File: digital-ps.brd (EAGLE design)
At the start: 73.7 x 50.8 mm, 85 parts, among them CON1 SWD_CON, IC1 STM32F334K8, IC2 MCP14700, IC3 7805, IC4 7805, IC5 3.3V, Q1 40V, Q2 40V, X1 12MHz

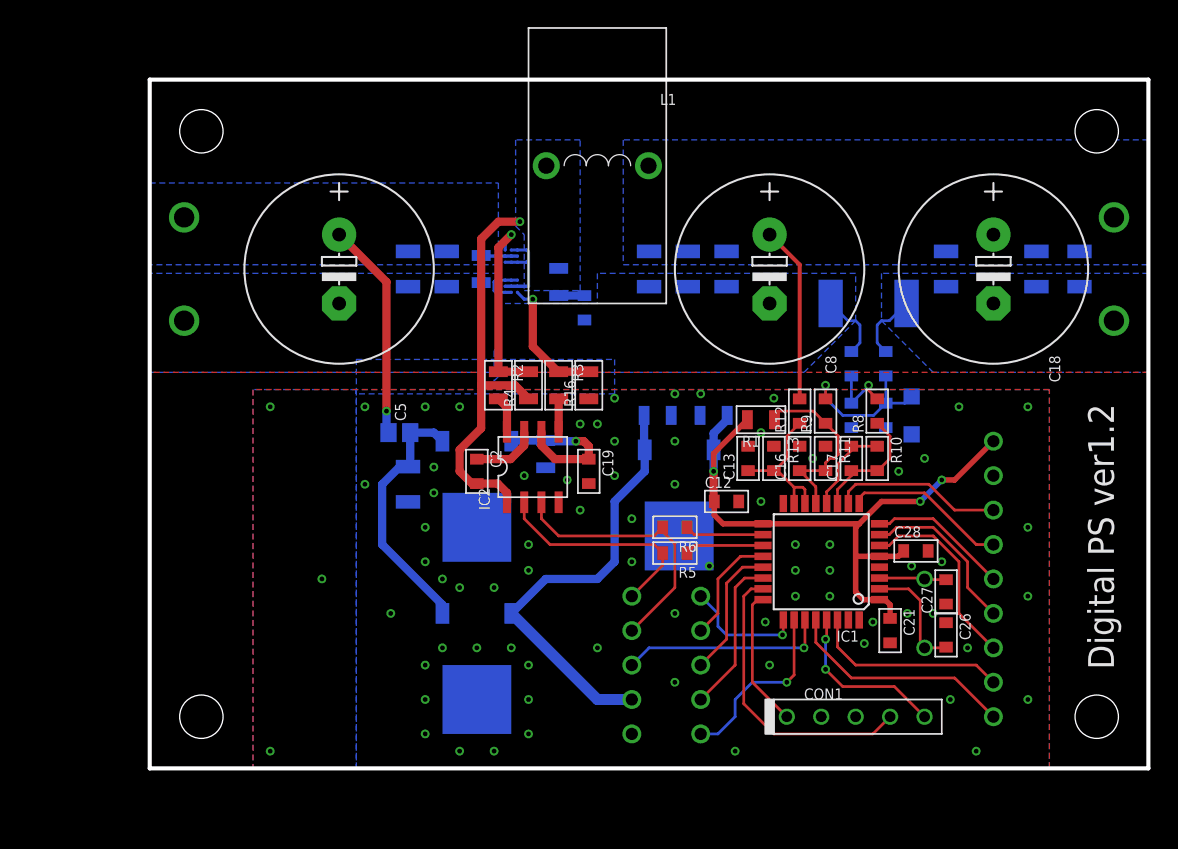
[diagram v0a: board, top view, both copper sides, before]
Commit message: 微修正
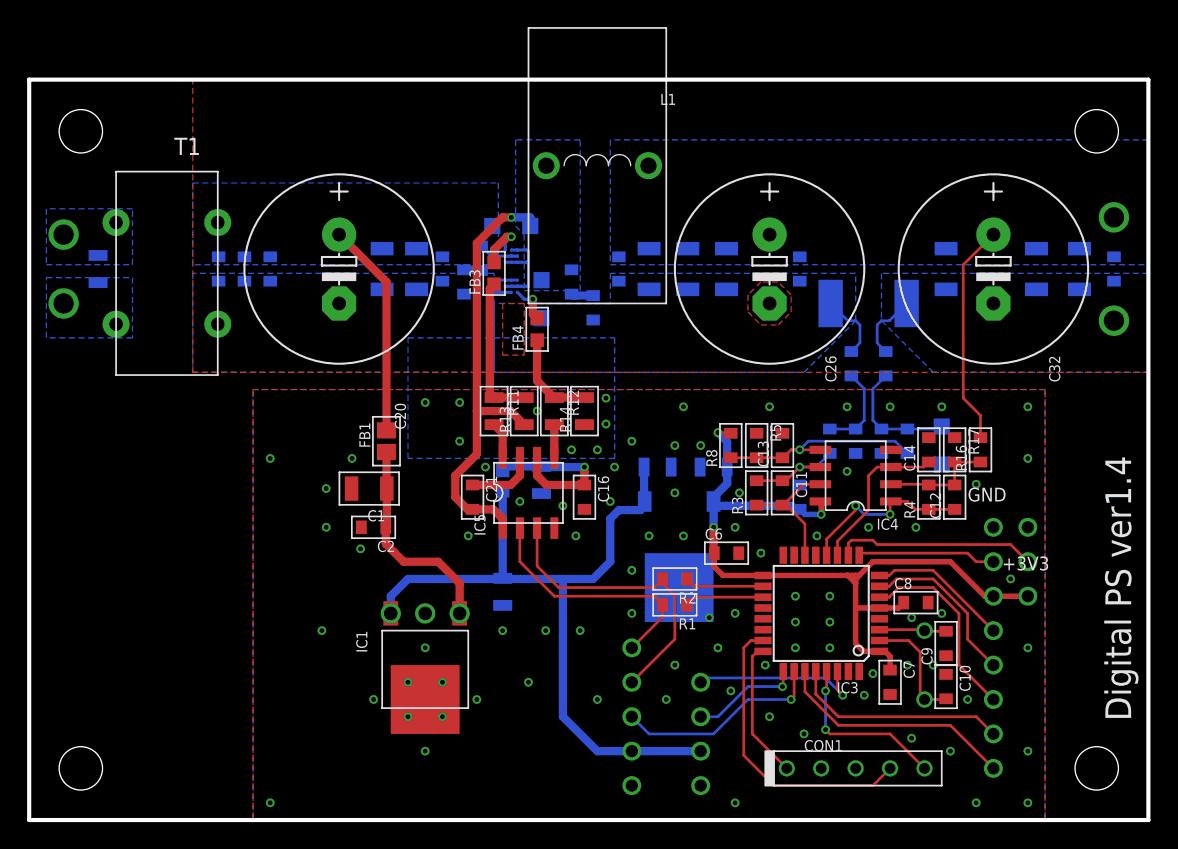
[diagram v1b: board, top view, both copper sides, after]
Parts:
- removed TP12: PA12, my_connector:TESTPIN
- removed TP13: PA11, my_connector:TESTPIN
- removed TP14: PA10, my_connector:TESTPIN
- added C30, C31, C33, C34: 10u, my_rcl:3225-2
- added C32: DNP, my_rcl:E5-13
- added C35, C36, C37, C39, C40: 1u, my_rcl:1608-2
- added C38: 0.1u, my_rcl:1608-2
- added C41: 1u, my_rcl:2012-2
- added D2, D3: SBD-1A2, my_rcl:SOD123
- added FB2: FB, my_rcl:1608-J
- added FB3, FB4: FB, my_rcl:1608-FB
- added R18: 10m, my_rcl:6432
- added R19: 2, my_rcl:1608-2
- added T1: COMMON_FILTER-SMALL, my_rcl:COMMON_FILTER__SMALL
- added TP24: +3V3, my_connector:TESTPIN
- added TP25, TP27: GND, my_connector:TESTPIN
- added TP26: +5V, my_connector:TESTPIN
- C1: device my_rcl:2012 -> my_rcl:3216
- C10, C9: value 10u -> 10p; device my_rcl:3216 -> my_rcl:1608
- C11: value 10u -> 1000p; device my_rcl:3216 -> my_rcl:1608
- C12: value 0.1u -> 1000p
- C15: value 1000p -> 10u; device my_rcl:1608 -> my_rcl:2012
- C16: value 1000p -> 0.1u
- C18: value DNP -> 1000p; device my_rcl:E5-13 -> my_rcl:1608
- C20: value 10u -> 1000u; device my_rcl:3216 -> my_rcl:E5-13
- C22, C23: device my_rcl:3216 -> my_rcl:3225-2
- C24: value 10u -> 1u; device my_rcl:3216 -> my_rcl:1608-2
- C25: value 10u -> 1n; device my_rcl:3216 -> my_rcl:1608-2
- C26: value 10p -> DNP; device my_rcl:1608 -> my_rcl:E5-13
- C27: value 10p -> 1u; device my_rcl:1608 -> my_rcl:1608-2
- C28: value 0.1u -> 10u; device my_rcl:1608 -> my_rcl:3225-2
- C29: value 1n -> 10u; device my_rcl:1608 -> my_rcl:3225-2
- C5: value 1000u -> 10u; device my_rcl:E5-13 -> my_rcl:2012
- C6: value 1u -> 0.1u; device my_rcl:2012 -> my_rcl:1608
- C7: value 10u -> 0.1u; device my_rcl:3216 -> my_rcl:1608
- C8: value DNP -> 0.1u; device my_rcl:E5-13 -> my_rcl:1608
- IC1: value STM32F334K8 -> 7805; device my_ic:TQFP32-08 -> my_ic:TO220-SOP-DUAL
- IC2: value MCP14700 -> 3.3V; device my_ic:SOP8 -> my_ic:P-HSIP3_2.30A
- IC3: value 7805 -> STM32F334K8; device my_ic:P-HSIP3_2.30A -> my_ic:TQFP32-08
- IC4: value 7805 -> OPA; device my_ic:P-HSIP3_2.30A -> my_ic:SOP8
- IC5: value 3.3V -> MCP14700; device my_ic:P-HSIP3_2.30A -> my_ic:SOP8
- Q1, Q2: value 40V -> EPC2052
- R1: value 1M -> 120; device my_rcl:2012 -> my_rcl:1608
- R10: value 10k -> 100
- R11, R12: value 10k -> 10; device my_rcl:1608 -> my_rcl:2012
- R13: value 1k -> 10k; device my_rcl:1608 -> my_rcl:2012
- R14: value 100 -> 10k; device my_rcl:1608 -> my_rcl:2012
- R15: value 100 -> 10; device my_rcl:1608 -> my_rcl:1608-2
- R16, R4: device my_rcl:2012 -> my_rcl:1608
- R17: value 10 -> 1k; device my_rcl:2012 -> my_rcl:1608
- R2: value 10 -> 120; device my_rcl:2012 -> my_rcl:1608
- R3: value 10 -> 10k; device my_rcl:2012 -> my_rcl:1608
- R5: value 120 -> 10k
- R6: value 120 -> 1k
- R7: value 40m -> 1k; device my_rcl:6432 -> my_rcl:1608
- R8: value 1k -> 1M
- R9: value 1k -> 100
- moved DR2 86.5 mm to (-5.08, 47.0)
- moved DR3 81.1 mm to (69.8, 0.00)
- moved C9 48.4 mm to (58.7, 9.21), flipped to the top, turned to 90 degrees
- moved C7 44.7 mm to (54.6, 6.35), flipped to the top
- moved C24 43.8 mm to (21.6, 36.8)
- moved C23 39.1 mm to (19.7, 36.8)
- moved C10 37.8 mm to (58.7, 6.03), flipped to the top
- moved C27 33.9 mm to (34.6, 36.8), flipped to the bottom, turned to 270 degrees
- moved C21 32.3 mm to (23.8, 20.0)
- moved R17 31.7 mm to (59.4, 23.5), flipped to the top, turned to 270 degrees
- moved R4 30.7 mm to (57.5, 20.0)
- moved C26 30.0 mm to (45.7, 36.8)
- moved IC4 29.7 mm to (52.1, 21.6), flipped to the top, turned to 90 degrees
- moved IC1 29.5 mm to (20.3, 11.4)
- moved R16 29.3 mm to (61.3, 23.5)
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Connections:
- removed net N$20: IC1.20, TP14.1
- removed net N$21: IC1.21, TP13.1
- removed net N$22: IC1.22, TP12.1
- removed net VCC: C20.1, FB1.2, IC3.1, IC4.1
- new net IN+: C41.1, T1.4, TP5.1
- new net IN-: C41.2, T1.1, TP6.1
- new net N$29: C11.1, IC4.6, R3.2, R6.1
- new net N$30: C12.1, IC3.12, IC4.1, R4.1
- new net N$31: C14.1, IC3.11, IC4.3
- new net N$32: FB3.1, R11.1, R13.2
- new net N$33: FB4.1, R12.1, R14.2
- new net N$34: C38.1, R19.1
- net +3V3: now also C19.1, C6.1, C7.1, C8.1, IC2.3, IC3.1, IC3.17, IC3.5, IC4.8, R8.2, TP24.1; no longer C12.1, C21.1, C28.1, IC1.1, IC1.17, IC1.5, IC5.3, R1.1
- net +5V: now also C5.1, FB2.1, IC1.3, IC1.6, IC2.1, TP26.1; no longer IC4.3, IC5.1
- net +5VP: now also C15.1, C16.1, FB2.2, IC5.6; no longer C1.1, C19.1, IC2.6, IC3.3
- net GND: now also C10.1, C15.2, C17.1, C18.2, C2.2, C20.-, C23.2, C24.2, C26.-, C27.2, C30.2, C35.2, C36.2, C37.2, C38.2, C39.2, C5.2, C8.2, C9.1, D3.1, IC1.2, IC1.5, IC2.2, IC3.16, IC3.31, IC3.32, IC4.4, IC5.4, R14.1, R17.1, R18.1, R5.1, R9.2, T1.2, TP25.1, TP27.1; no longer C10.2, C12.2, C15.1, C20.2, C21.2, C26.1, C27.1, C5.-, C8.-, C9.2, IC1.16, IC1.31, IC1.32, IC2.4, IC3.2, IC4.2, IC5.2, R11.1, R13.1, R14.2, R16.1, R7.1, TP6.1
- net N$1: now also IC3.18, R2.1; no longer IC1.18, R6.1
- net N$10: now also FB4.2; no longer R16.2, R3.1
- net N$11: now also C18.1, R10.1, R7.2; no longer C14.1, R15.1, R9.2
- net N$12: now also IC5.5, R12.2; no longer IC2.5, R3.2
- net N$13: now also IC3.9; no longer IC1.9
- net N$14: now also IC3.10; no longer IC1.10
- net N$15: now also IC3.6; no longer IC1.6
- net N$16: now also IC3.7; no longer IC1.7
- net N$17: now also IC3.8; no longer IC1.8
- net N$18: now also IC3.30; no longer IC1.30
- net N$19: now also IC3.28; no longer IC1.28
- net N$2: now also IC3.19, R1.1; no longer IC1.19, R5.1
- net N$23: now also IC3.27; no longer IC1.27
- net N$24: now also C10.2, IC3.2; no longer C26.2, IC1.2
- net N$25: now also C9.2, IC3.3; no longer C27.2, IC1.3
- net N$26: now also IC3.26; no longer IC1.26
- net N$27: now also IC3.25; no longer IC1.25
- net N$28: now also C25.1, R15.1; no longer C29.1, R17.1
- net N$3: now also C11.2, IC3.14, IC4.7, R3.1; no longer C17.2, IC1.12, R10.1
- net N$4: now also C1.1, C2.1, FB1.2, IC1.1, IC1.4; no longer C17.1, IC1.11, R10.2, R8.1
- net N$5: now also C13.1, IC4.5, R5.2, R7.1, R8.1; no longer C16.1, IC1.13, R1.2, R11.2, R9.1
- net N$6: now also IC5.8, R11.2; no longer IC2.8, R2.2
- net N$7: now also C21.1, IC5.7; no longer C2.1, IC2.7
- net N$8: now also C17.2, R6.2, R9.1; no longer C15.2, R14.1, R8.2
- net N$9: now also FB3.2; no longer R2.1, R4.2
- net OUT+: now also C26.+, C27.1, C28.1, C29.1, C30.1, C31.1, C32.+, C33.1, C34.1, C39.1, C40.1, R16.2; no longer C10.1, C11.1, C18.+, C22.1, C23.1, C24.1, C25.1, C8.+, R12.2
- net OUT-: now also C31.2, C32.-, C33.2, C34.2, C40.2, R10.2, R18.2; no longer C11.2, C18.-, C23.2, C24.2, R15.2, R7.2
- net PWMH: now also IC5.2, R1.2; no longer IC2.2, R5.2
- net PWML: now also IC5.3, R2.2; no longer IC2.3, R6.2
- net SW: now also C21.2, D2.1, D3.2, IC5.1, R13.1, R15.2; no longer C2.2, IC2.1, R17.2, R4.1
- net SWCLK: now also IC3.24; no longer IC1.24
- net SWDIO: now also IC3.23; no longer IC1.23
- net UART_TX: now also IC3.29; no longer IC1.29
- net VFB: now also C12.2, IC4.2, R16.1, R17.2, R4.2; no longer C13.1, IC1.14, IC1.15, R12.1, R13.2
- net VP: now also C20.+, C22.1, C23.1, C24.1, C35.1, C36.1, C37.1, D2.2, R19.2, T1.3; no longer C5.+, C6.1, C7.1, C9.1, TP5.1
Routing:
- net +5V: track 32.5 -> 55.4 mm
- net VCC: track 19.0 -> 0.00 mm
- net N$30: track 0.00 -> 13.3 mm, vias 0 -> 2
- net N$31: track 0.00 -> 11.7 mm
- net N$22: track 11.7 -> 0.00 mm
- net N$32: track 0.00 -> 10.8 mm
- net +3V3: track 49.1 -> 59.7 mm
- net N$9: track 14.1 -> 3.78 mm
- net N$21: track 10.0 -> 0.00 mm
- net N$20: track 8.36 -> 0.00 mm
- net N$29: track 0.00 -> 7.76 mm, vias 0 -> 1
- net N$33: track 0.00 -> 7.01 mm
- net N$10: track 9.74 -> 2.90 mm
- net N$4: track 9.07 -> 15.7 mm
- net SW: track 37.3 -> 40.9 mm
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- added copper zone on layer 16, net IN+
- added copper zone on layer 16, net IN-
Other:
- board size 73.7 x 50.8 mm -> 82.5 x 54.6 mm
- board text added: "Digital PS ver1.4"
- board text removed: "Digital PS ver1.2"
